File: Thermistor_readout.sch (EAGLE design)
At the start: 25 parts, among them Q1 BC550C, U1 TI_NATIONAL_SEMICONDUCTOR_LF3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, U2 TI_NATIONAL_SEMICONDUCTOR_LF3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, U3 ANALOG_DEVICES_ADG725BSUZANAL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, U4 TI_NATIONAL_SEMICONDUCTOR_LF3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

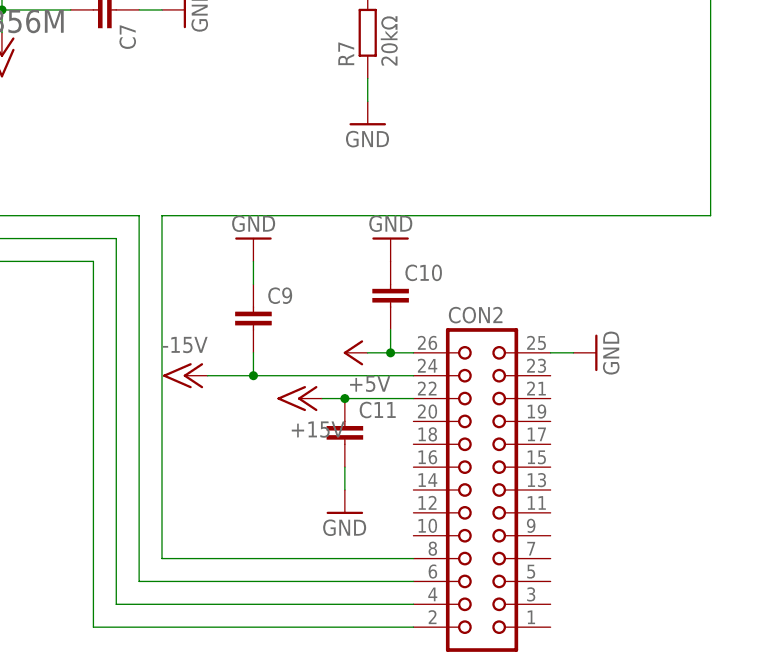
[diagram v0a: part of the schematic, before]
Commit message: Internal_switch_v1.1
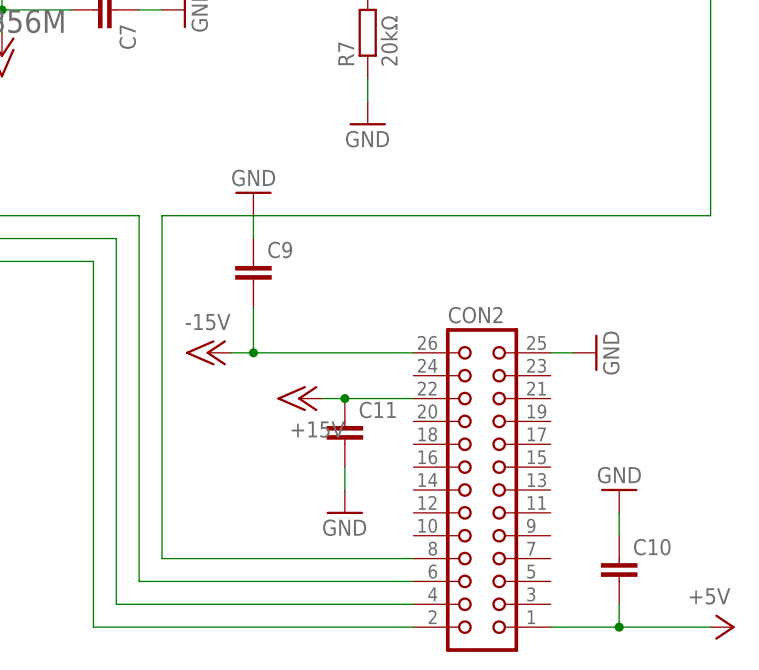
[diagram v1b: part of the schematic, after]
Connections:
- net +5V: now also CON2.1; no longer CON2.26
- net -15V: now also CON2.26; no longer CON2.24
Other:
- moved on the sheet: C10, C9
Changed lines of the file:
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@@
 <instance part="GND3" gate="1" x="53.34" y="60.96"/>
 <instance part="GND4" gate="1" x="172.72" y="58.42"/>
-<instance part="P+1" gate="1" x="170.18" y="33.02" rot="R90"/>
+<instance part="P+1" gate="1" x="213.36" y="2.54" rot="R270"/>
 <instance part="P+2" gate="1" x="35.56" y="152.4"/>
 <instance part="P+4" gate="1" x="66.04" y="38.1" rot="R90"/>
@@
 <instance part="GND12" gate="1" x="152.4" y="114.3" rot="R90"/>
 <instance part="P+7" gate="1" x="165.1" y="27.94" rot="R90"/>
-<instance part="P-4" gate="1" x="152.4" y="30.48" rot="R270"/>
+<instance part="P-4" gate="1" x="154.94" y="33.02" rot="R270"/>
 <instance part="P+9" gate="1" x="127" y="147.32"/>
 <instance part="P+10" gate="1" x="177.8" y="124.46"/>
@@
 <instance part="GND14" gate="1" x="152.4" y="71.12" rot="R90"/>
 <instance part="RE" gate="G$1" x="53.34" y="71.12" rot="R90"/>
-<instance part="GND15" gate="1" x="175.26" y="45.72" rot="R180"/>
-<instance part="GND16" gate="1" x="160.02" y="45.72" rot="R180"/>
+<instance part="GND15" gate="1" x="200.66" y="17.78" rot="R180"/>
+<instance part="GND16" gate="1" x="160.02" y="50.8" rot="R180"/>
 <instance part="GND17" gate="1" x="170.18" y="15.24"/>
-<instance part="C9" gate="G$1" x="160.02" y="38.1"/>
-<instance part="C10" gate="G$1" x="175.26" y="40.64"/>
+<instance part="C9" gate="G$1" x="160.02" y="43.18"/>
+<instance part="C10" gate="G$1" x="200.66" y="10.16"/>
 <instance part="C11" gate="G$1" x="170.18" y="25.4"/>
 </instances>
@@
 <pinref part="GND16" gate="1" pin="GND"/>
 <pinref part="C9" gate="G$1" pin="1"/>
-<wire x1="160.02" y1="40.64" x2="160.02" y2="43.18" width="0.1524" layer="91"/>
+<wire x1="160.02" y1="45.72" x2="160.02" y2="48.26" width="0.1524" layer="91"/>
 </segment>
 <segment>
 <pinref part="GND15" gate="1" pin="GND"/>
 <pinref part="C10" gate="G$1" pin="1"/>
+<wire x1="200.66" y1="15.24" x2="200.66" y2="12.7" width="0.1524" layer="91"/>
 </segment>
 <segment>
@@
 </segment>
 <segment>
+<pinref part="CON2" gate="A" pin="1"/>
 <pinref part="P+1" gate="1" pin="+5V"/>
-<pinref part="CON2" gate="A" pin="26"/>
-<wire x1="172.72" y1="33.02" x2="175.26" y2="33.02" width="0.1524" layer="91"/>
+<wire x1="193.04" y1="2.54" x2="200.66" y2="2.54" width="0.1524" layer="91"/>
 <pinref part="C10" gate="G$1" pin="2"/>
-<wire x1="175.26" y1="33.02" x2="177.8" y2="33.02" width="0.1524" layer="91"/>
-<wire x1="175.26" y1="33.02" x2="175.26" y2="35.56" width="0.1524" layer="91"/>
-<junction x="175.26" y="33.02"/>
+<wire x1="200.66" y1="2.54" x2="210.82" y2="2.54" width="0.1524" layer="91"/>
+<wire x1="200.66" y1="2.54" x2="200.66" y2="5.08" width="0.1524" layer="91"/>
+<junction x="200.66" y="2.54"/>
 </segment>
 </net>
@@
 </segment>
 <segment>
+<pinref part="CON2" gate="A" pin="26"/>
 <pinref part="P-4" gate="1" pin="-15V"/>
-<pinref part="CON2" gate="A" pin="24"/>
-<wire x1="154.94" y1="30.48" x2="160.02" y2="30.48" width="0.1524" layer="91"/>
+<wire x1="157.48" y1="33.02" x2="160.02" y2="33.02" width="0.1524" layer="91"/>
 <pinref part="C9" gate="G$1" pin="2"/>
-<wire x1="160.02" y1="30.48" x2="177.8" y2="30.48" width="0.1524" layer="91"/>
-<wire x1="160.02" y1="30.48" x2="160.02" y2="33.02" width="0.1524" layer="91"/>
-<junction x="160.02" y="30.48"/>
-</segment>
-</net>
+<wire x1="160.02" y1="33.02" x2="177.8" y2="33.02" width="0.1524" layer="91"/>
+<wire x1="160.02" y1="38.1" x2="160.02" y2="33.02" width="0.1524" layer="91"/>
+<junction x="160.02" y="33.02"/>
+</segment>
+</net>
